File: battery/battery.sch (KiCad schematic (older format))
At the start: 53 parts, among them J1 batt_1, J2 batt_2, J3 batt_3, J4 batt_4, J5 reed_switch, J6 toPcb+, J7 toPcb-, J8 on_signal, Q1 batt1_sw, Q2 batt2_sw, Q3 batt3_sw, Q4 batt4_sw, Q5 BC817-25, U1 LM1117-5.0, U2 LTV-817S

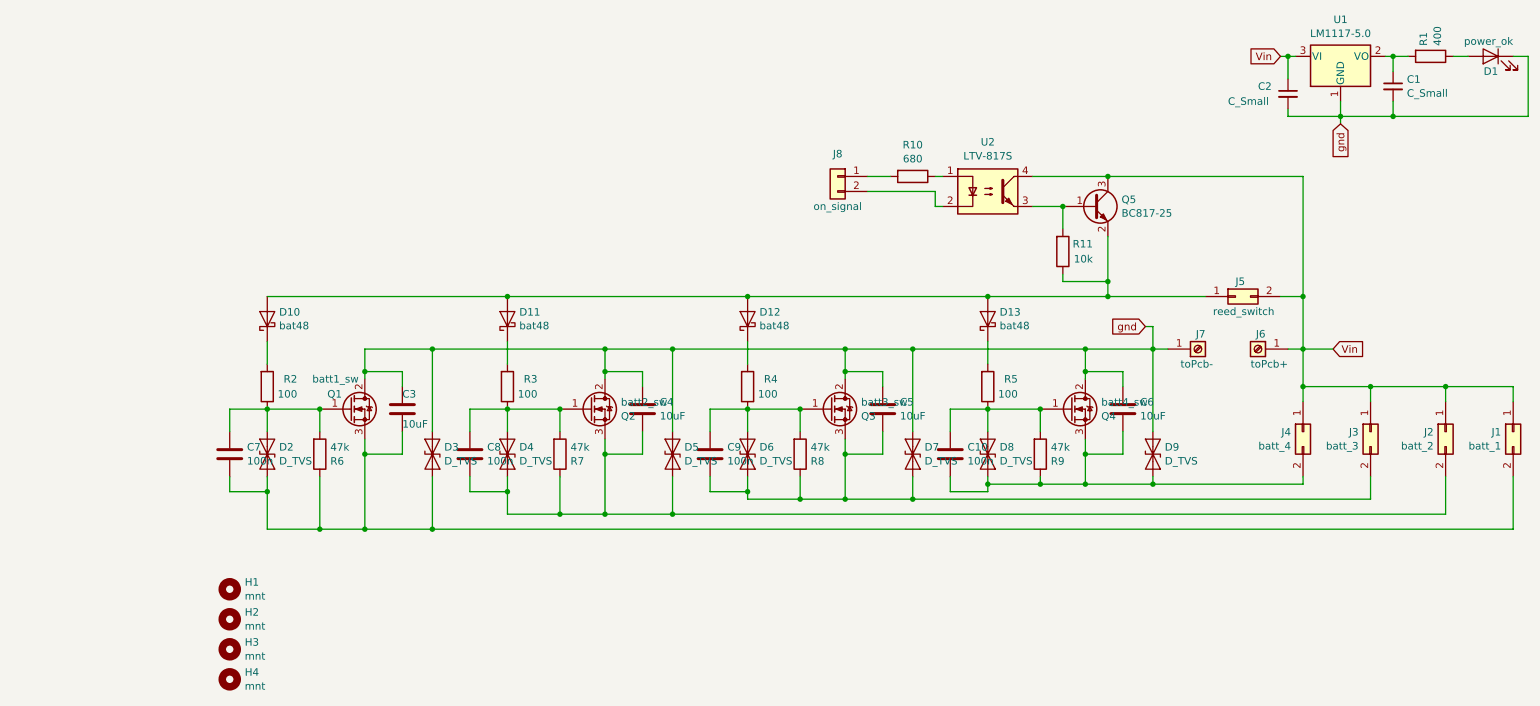
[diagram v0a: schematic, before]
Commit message: visual fix
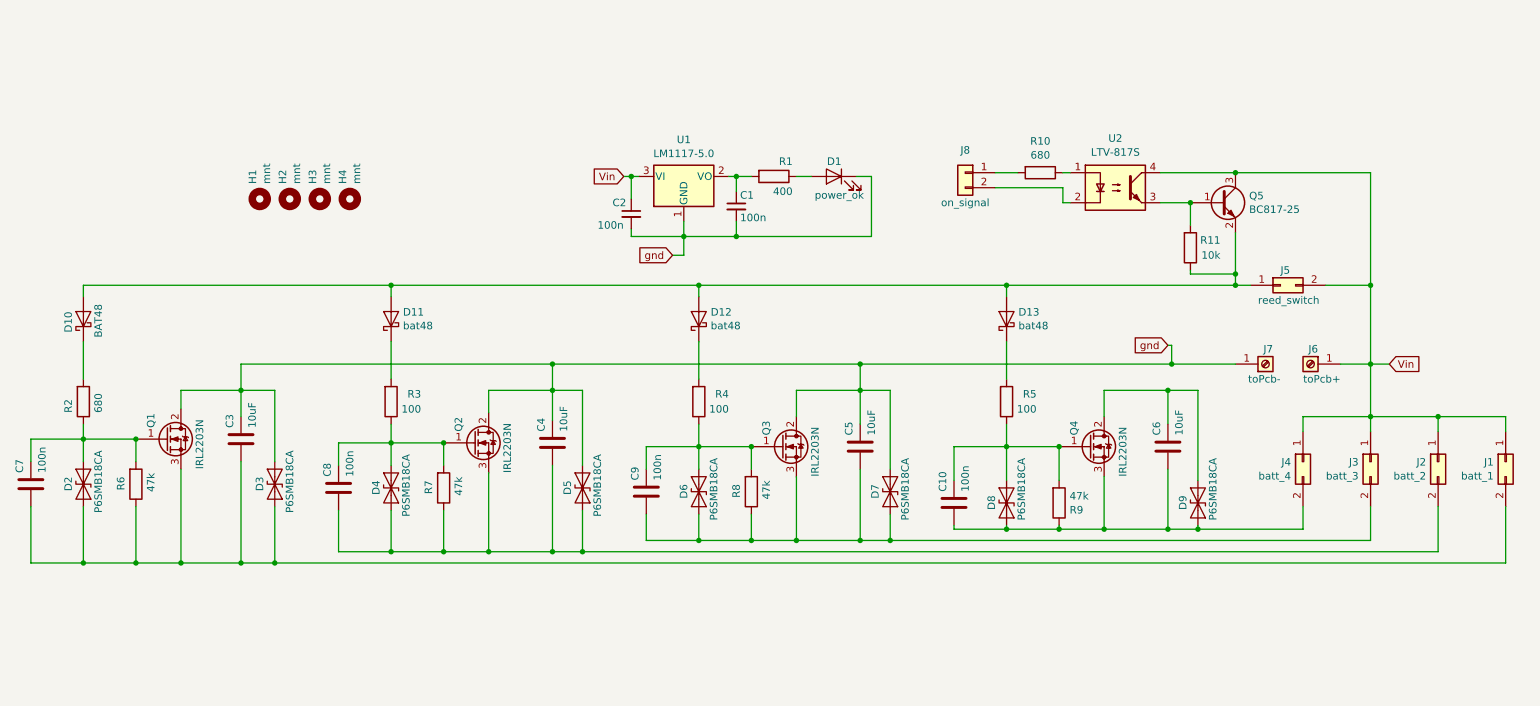
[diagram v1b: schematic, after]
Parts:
- C1, C2: value C_Small -> 100n
- D10: value bat48 -> BAT48
- D2, D3, D4, D5, D6, D7, D8, D9: value D_TVS -> P6SMB18CA
- Q1: value batt1_sw -> IRL2203N
- Q2: value batt2_sw -> IRL2203N
- Q3: value batt3_sw -> IRL2203N
- Q4: value batt4_sw -> IRL2203N
- R2: value 100 -> 680
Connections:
- net gnd: no longer C6.1, D9.1 (A1), Q4.2 (D)
- new net: C6.1, D9.1 (A1), Q4.2 (D)
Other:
- moved on the sheet: C1, C10, C2, C3, C4, C5, C6, C7, C8, C9, D1, D10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
